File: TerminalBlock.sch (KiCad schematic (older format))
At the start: 2 parts, among them P4 12 Pin Terminal Block, P5 3 Pin TB

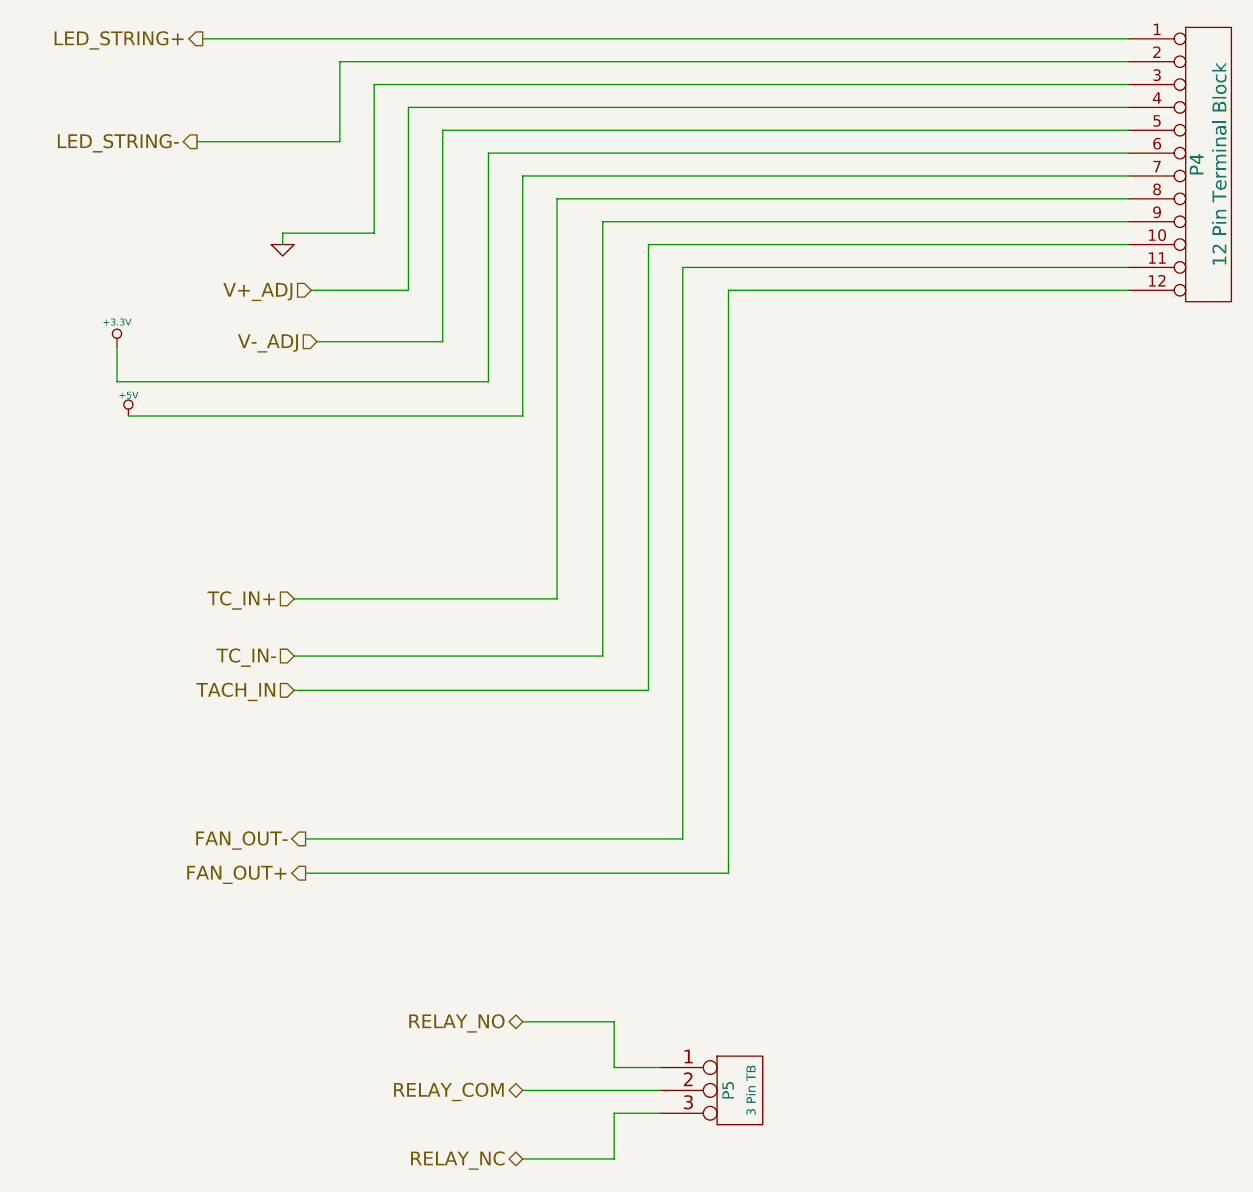
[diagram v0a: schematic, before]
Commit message: Layout Work Session 2
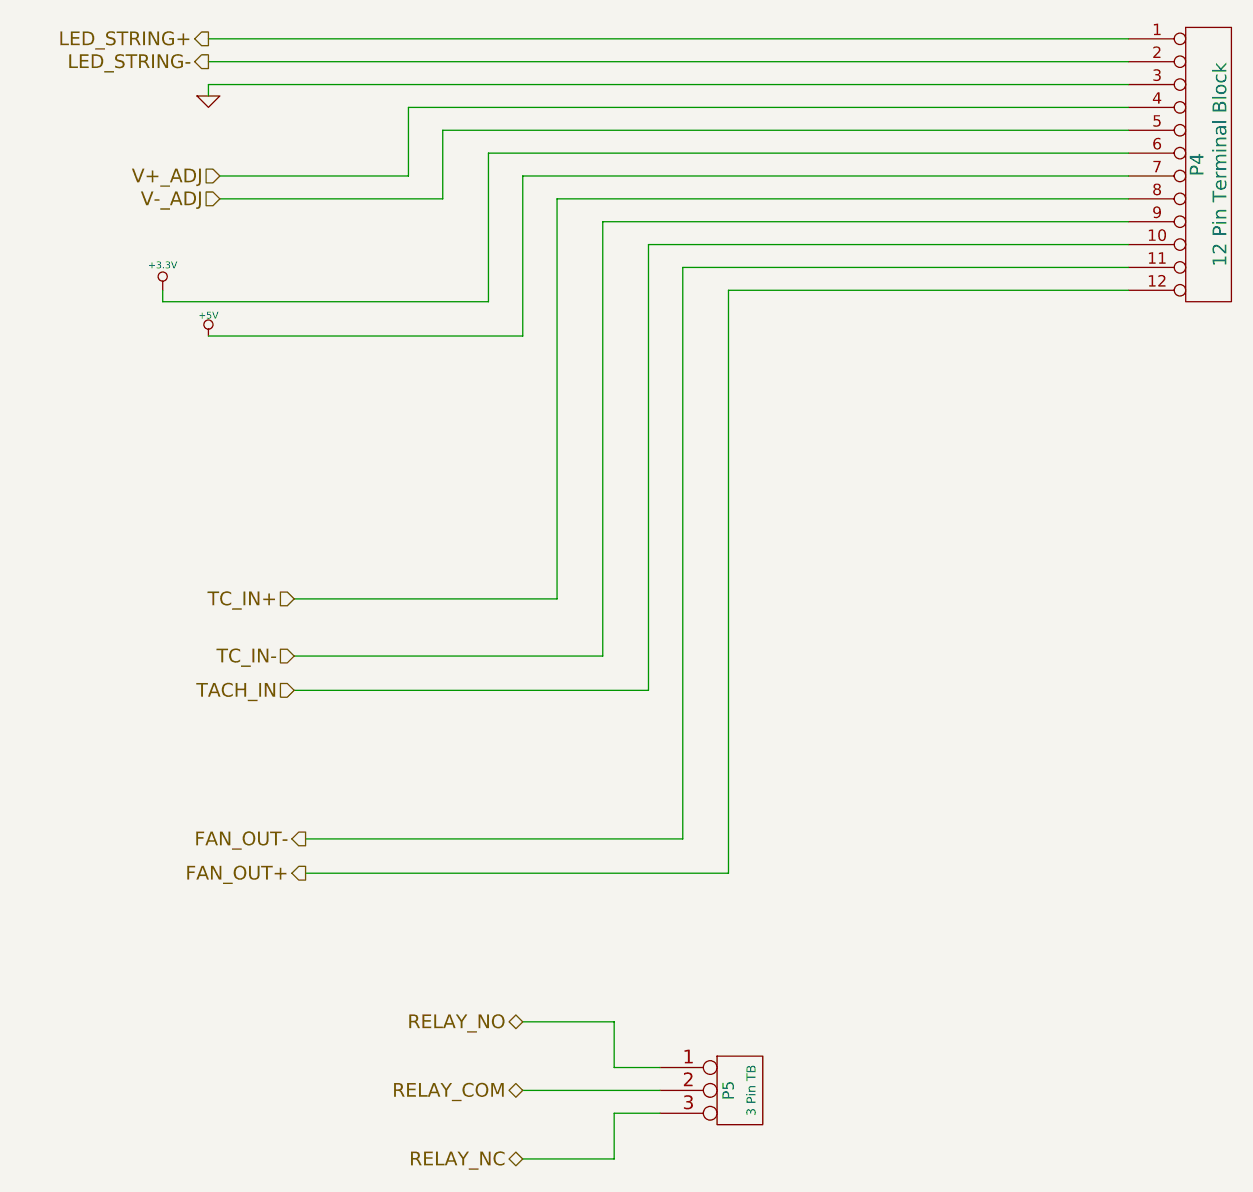
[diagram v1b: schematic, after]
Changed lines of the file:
@@
 LIBS:valves
 LIBS:BenchBuddy
+LIBS:arduino_shieldsNCL
 LIBS:BenchBuddy-cache
 EELAYER 24 0
@@
 Comment4 ""
 $EndDescr
-Text HLabel 1925 2000 0    60   Input ~ 0
+Text HLabel 1525 1500 0    60   Input ~ 0
 V+_ADJ
-Text HLabel 1950 2225 0    60   Input ~ 0
+Text HLabel 1525 1600 0    60   Input ~ 0
 V-_ADJ
 Text HLabel 1900 4550 0    60   Output ~ 0
@@
 Text HLabel 1850 3750 0    60   Input ~ 0
 TACH_IN
-Text HLabel 1450 900  0    60   Output ~ 0
+Text HLabel 1475 900  0    60   Output ~ 0
 LED_STRING+
-Text HLabel 1425 1350 0    60   Output ~ 0
+Text HLabel 1475 1000 0    60   Output ~ 0
 LED_STRING-
 Text HLabel 1850 3350 0    60   Input ~ 0
@@
 RELAY_NC
 $Comp
-L +3.3V #PWR47
+L +3.3V #PWR041
 U 1 1 523FFDA7
-P 1075 2250
-F 0 "#PWR47" H 1075 2210 30  0001 C CNN
-F 1 "+3.3V" H 1075 2360 30  0000 C CNN
-F 2 "~" H 1075 2250 60  0000 C CNN
-F 3 "~" H 1075 2250 60  0000 C CNN
-	1    1075 2250
+P 1275 2000
+F 0 "#PWR041" H 1275 1960 30  0001 C CNN
+F 1 "+3.3V" H 1275 2110 30  0000 C CNN
+F 2 "~" H 1275 2000 60  0000 C CNN
+F 3 "~" H 1275 2000 60  0000 C CNN
+	1    1275 2000
 	1    0    0    -1
 $EndComp
 $Comp
-L +5V #PWR48
+L +5V #PWR042
 U 1 1 523FFDB6
-P 1125 2550
-F 0 "#PWR48" H 1125 2640 20  0001 C CNN
-F 1 "+5V" H 1125 2640 30  0000 C CNN
-F 2 "~" H 1125 2550 60  0000 C CNN
-F 3 "~" H 1125 2550 60  0000 C CNN
-	1    1125 2550
+P 1475 2200
+F 0 "#PWR042" H 1475 2290 20  0001 C CNN
+F 1 "+5V" H 1475 2290 30  0000 C CNN
+F 2 "~" H 1475 2200 60  0000 C CNN
+F 3 "~" H 1475 2200 60  0000 C CNN
+	1    1475 2200
 	1    0    0    -1
 $EndComp
@@
 $EndComp
 Wire Wire Line
-	1450 900  5500 900
+	1475 1000 5500 1000
 Wire Wire Line
-	1425 1350 2050 1350
+	1475 1100 5500 1100
 Wire Wire Line
-	2050 1350 2050 1000
+	1475 1100 1475 1150
 Wire Wire Line
-	2050 1000 5500 1000
-Wire Wire Line
-	2200 1100 5500 1100
-Wire Wire Line
-	2200 1100 2200 1750
-Wire Wire Line
-	1800 1750 1800 1800
-Wire Wire Line
-	2350 2000 2350 1200
+	2350 1500 2350 1200
 Wire Wire Line
 	2350 1200 5500 1200
@@
 	5500 1300 2500 1300
 Wire Wire Line
-	2500 1300 2500 2225
+	2500 1300 2500 1600
 Wire Wire Line
-	2700 2400 2700 1400
+	2700 2050 2700 1400
 Wire Wire Line
 	2700 1400 5500 1400
@@
 	1850 3750 3400 3750
 Wire Wire Line
-	2850 2550 2850 1500
+	2850 2200 2850 1500
 Wire Wire Line
 	2850 1500 5500 1500
@@
 	3250 5800 2850 5800
 Wire Wire Line
-	1125 2550 2850 2550
+	1475 2200 2850 2200
 Wire Wire Line
-	2700 2400 1075 2400
+	2700 2050 1275 2050
 Wire Wire Line
-	1075 2400 1075 2250
+	1275 2050 1275 2000
 Wire Wire Line
-	2500 2225 1950 2225
+	2500 1600 1525 1600
 Wire Wire Line
-	1925 2000 2350 2000
+	1525 1500 2350 1500
 $Comp
-L GND #PWR49
+L GND #PWR043
 U 1 1 523FFDC5
-P 1800 1800
-F 0 "#PWR49" H 1800 1800 30  0001 C CNN
-F 1 "GND" H 1800 1730 30  0001 C CNN
-F 2 "~" H 1800 1800 60  0000 C CNN
-F 3 "~" H 1800 1800 60  0000 C CNN
-	1    1800 1800
+P 1475 1150
+F 0 "#PWR043" H 1475 1150 30  0001 C CNN
+F 1 "GND" H 1475 1080 30  0001 C CNN
+F 2 "~" H 1475 1150 60  0000 C CNN
+F 3 "~" H 1475 1150 60  0000 C CNN
+	1    1475 1150
 	1    0    0    -1
 $EndComp
 Wire Wire Line
-	2200 1750 1800 1750
-Wire Wire Line
-	1750 900  1750 900
+	1475 900  5500 900
 $EndSCHEMATC

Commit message: Layout Work Session 4
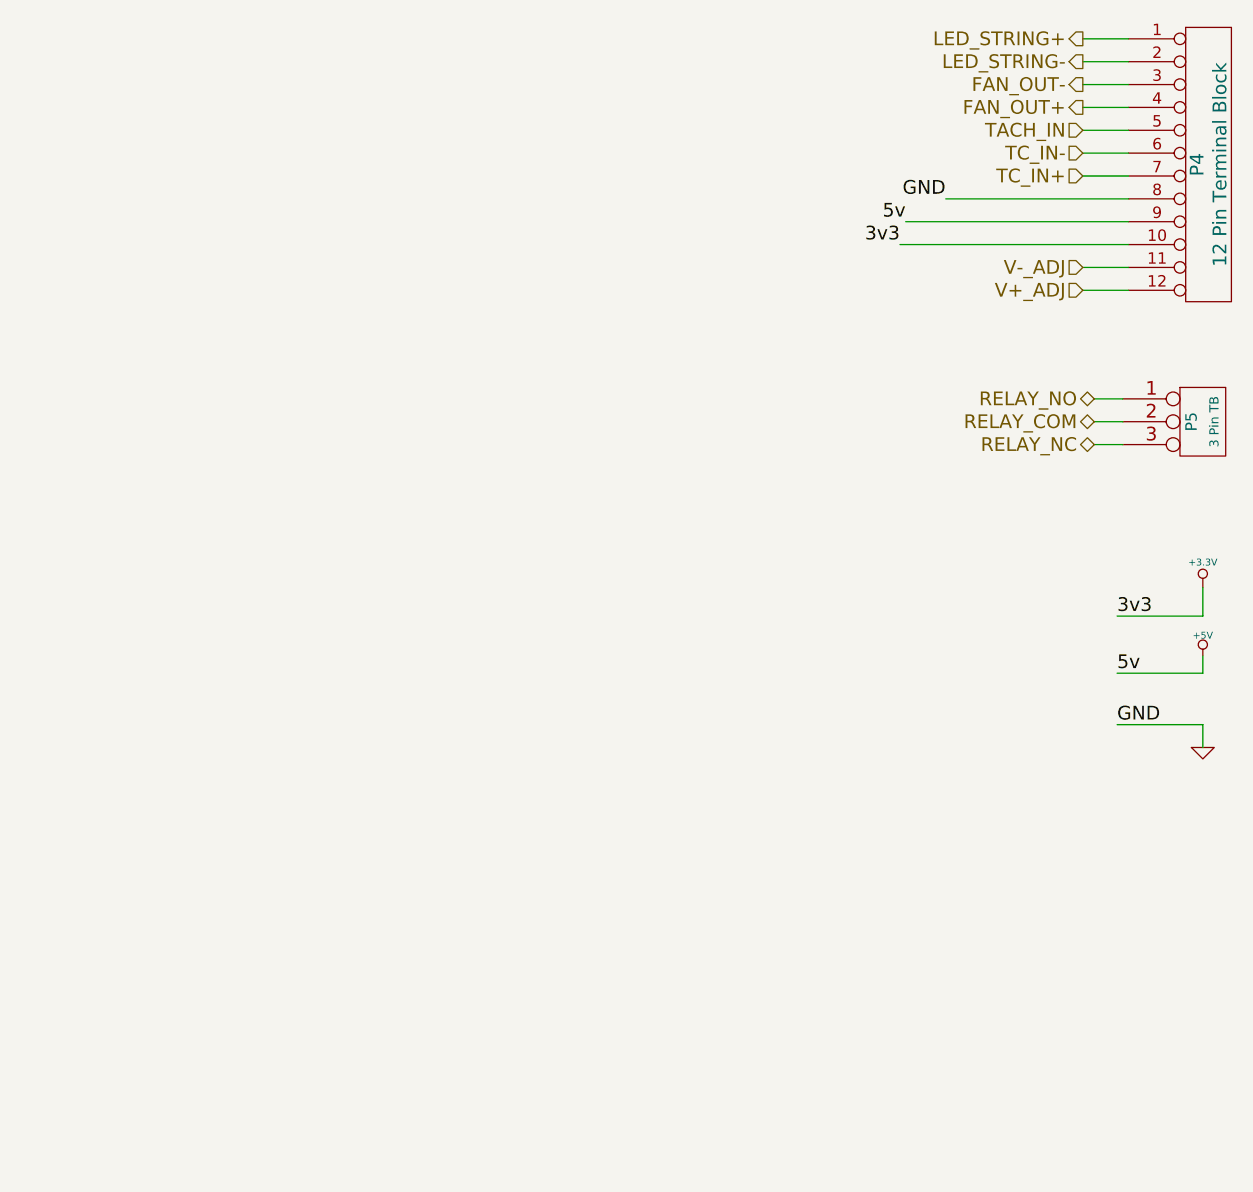
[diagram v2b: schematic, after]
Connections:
- net +3.3V: now also P4.10 (P10); no longer P4.6 (P6)
- net +5V: now also P4.9 (P9); no longer P4.7 (P7)
- net FAN_OUT+: now also P4.4 (P4); no longer P4.12 (P12)
- net FAN_OUT-: now also P4.3 (P3); no longer P4.11 (P11)
- net GND: now also P4.8 (P8); no longer P4.3 (P3)
- net TACH_IN: now also P4.5 (P5); no longer P4.10 (P10)
- net TC_IN+: now also P4.7 (P7); no longer P4.8 (P8)
- net TC_IN-: now also P4.6 (P6); no longer P4.9 (P9)
- net V+_ADJ: now also P4.12 (P12); no longer P4.4 (P4)
- net V-_ADJ: now also P4.11 (P11); no longer P4.5 (P5)
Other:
- moved on the sheet: P5
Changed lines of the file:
@@
 Comment4 ""
 $EndDescr
-Text HLabel 1525 1500 0    60   Input ~ 0
+Text HLabel 5300 2000 0    60   Input ~ 0
 V+_ADJ
-Text HLabel 1525 1600 0    60   Input ~ 0
+Text HLabel 5300 1900 0    60   Input ~ 0
 V-_ADJ
-Text HLabel 1900 4550 0    60   Output ~ 0
+Text HLabel 5300 1200 0    60   Output ~ 0
 FAN_OUT+
-Text HLabel 1900 4400 0    60   Output ~ 0
+Text HLabel 5300 1100 0    60   Output ~ 0
 FAN_OUT-
-Text HLabel 1850 3750 0    60   Input ~ 0
+Text HLabel 5300 1300 0    60   Input ~ 0
 TACH_IN
-Text HLabel 1475 900  0    60   Output ~ 0
+Text HLabel 5300 900  0    60   Output ~ 0
 LED_STRING+
-Text HLabel 1475 1000 0    60   Output ~ 0
+Text HLabel 5300 1000 0    60   Output ~ 0
 LED_STRING-
-Text HLabel 1850 3350 0    60   Input ~ 0
+Text HLabel 5300 1500 0    60   Input ~ 0
 TC_IN+
-Text HLabel 1850 3600 0    60   Input ~ 0
+Text HLabel 5300 1400 0    60   Input ~ 0
 TC_IN-
-Text HLabel 2850 5500 0    60   BiDi ~ 0
+Text HLabel 5350 2575 0    60   BiDi ~ 0
 RELAY_COM
-Text HLabel 2850 5200 0    60   BiDi ~ 0
+Text HLabel 5350 2475 0    60   BiDi ~ 0
 RELAY_NO
-Text HLabel 2850 5800 0    60   BiDi ~ 0
+Text HLabel 5350 2675 0    60   BiDi ~ 0
 RELAY_NC
 $Comp
-L +3.3V #PWR041
+L +3.3V #PWR038
 U 1 1 523FFDA7
-P 1275 2000
-F 0 "#PWR041" H 1275 1960 30  0001 C CNN
-F 1 "+3.3V" H 1275 2110 30  0000 C CNN
-F 2 "~" H 1275 2000 60  0000 C CNN
-F 3 "~" H 1275 2000 60  0000 C CNN
-	1    1275 2000
+P 5825 3300
+F 0 "#PWR038" H 5825 3260 30  0001 C CNN
+F 1 "+3.3V" H 5825 3410 30  0000 C CNN
+F 2 "~" H 5825 3300 60  0000 C CNN
+F 3 "~" H 5825 3300 60  0000 C CNN
+	1    5825 3300
 	1    0    0    -1
 $EndComp
 $Comp
-L +5V #PWR042
+L +5V #PWR039
 U 1 1 523FFDB6
-P 1475 2200
-F 0 "#PWR042" H 1475 2290 20  0001 C CNN
-F 1 "+5V" H 1475 2290 30  0000 C CNN
-F 2 "~" H 1475 2200 60  0000 C CNN
-F 3 "~" H 1475 2200 60  0000 C CNN
-	1    1475 2200
+P 5825 3600
+F 0 "#PWR039" H 5825 3690 20  0001 C CNN
+F 1 "+5V" H 5825 3690 30  0000 C CNN
+F 2 "~" H 5825 3600 60  0000 C CNN
+F 3 "~" H 5825 3600 60  0000 C CNN
+	1    5825 3600
 	1    0    0    -1
 $EndComp
@@
 	1    0    0    -1
 $EndComp
-Wire Wire Line
-	1475 1000 5500 1000
-Wire Wire Line
-	1475 1100 5500 1100
-Wire Wire Line
-	1475 1100 1475 1150
-Wire Wire Line
-	2350 1500 2350 1200
-Wire Wire Line
-	2350 1200 5500 1200
-Wire Wire Line
-	5500 1300 2500 1300
-Wire Wire Line
-	2500 1300 2500 1600
-Wire Wire Line
-	2700 2050 2700 1400
-Wire Wire Line
-	2700 1400 5500 1400
-Wire Wire Line
-	1850 3350 3000 3350
-Wire Wire Line
-	1850 3600 3200 3600
-Wire Wire Line
-	1850 3750 3400 3750
-Wire Wire Line
-	2850 2200 2850 1500
-Wire Wire Line
-	2850 1500 5500 1500
-Wire Wire Line
-	5500 1600 3000 1600
-Wire Wire Line
-	3000 1600 3000 3350
-Wire Wire Line
-	3200 3600 3200 1700
-Wire Wire Line
-	3200 1700 5500 1700
-Wire Wire Line
-	5500 1800 3400 1800
-Wire Wire Line
-	3400 1800 3400 3750
-Wire Wire Line
-	1900 4400 3550 4400
-Wire Wire Line
-	3550 4400 3550 1900
-Wire Wire Line
-	3550 1900 5500 1900
-Wire Wire Line
-	5500 2000 3750 2000
-Wire Wire Line
-	3750 2000 3750 4550
-Wire Wire Line
-	3750 4550 1900 4550
 $Comp
 L CONN_3 P5
 U 1 1 5258AA07
-P 3800 5500
-F 0 "P5" V 3750 5500 50  0000 C CNN
-F 1 "3 Pin TB" V 3850 5500 40  0000 C CNN
-F 2 "" H 3800 5500 60  0000 C CNN
-F 3 "" H 3800 5500 60  0000 C CNN
-F 4 "Phoenix" H 3800 5500 60  0001 C CNN "MFG Name"
-F 5 "1935174" H 3800 5500 60  0001 C CNN "MFG Part Number"
-	1    3800 5500
+P 5825 2575
+F 0 "P5" V 5775 2575 50  0000 C CNN
+F 1 "3 Pin TB" V 5875 2575 40  0000 C CNN
+F 2 "" H 5825 2575 60  0000 C CNN
+F 3 "" H 5825 2575 60  0000 C CNN
+F 4 "Phoenix" H 5825 2575 60  0001 C CNN "MFG Name"
+F 5 "1935174" H 5825 2575 60  0001 C CNN "MFG Part Number"
+	1    5825 2575
 	1    0    0    -1
 $EndComp
 Wire Wire Line
-	3450 5500 2850 5500
-Wire Wire Line
-	2850 5200 3250 5200
-Wire Wire Line
-	3250 5200 3250 5400
-Wire Wire Line
-	3250 5400 3450 5400
-Wire Wire Line
-	3450 5600 3250 5600
-Wire Wire Line
-	3250 5600 3250 5800
-Wire Wire Line
-	3250 5800 2850 5800
-Wire Wire Line
-	1475 2200 2850 2200
-Wire Wire Line
-	2700 2050 1275 2050
-Wire Wire Line
-	1275 2050 1275 2000
-Wire Wire Line
-	2500 1600 1525 1600
-Wire Wire Line
-	1525 1500 2350 1500
+	5475 2575 5350 2575
 $Comp
-L GND #PWR043
+L GND #PWR040
 U 1 1 523FFDC5
-P 1475 1150
-F 0 "#PWR043" H 1475 1150 30  0001 C CNN
-F 1 "GND" H 1475 1080 30  0001 C CNN
-F 2 "~" H 1475 1150 60  0000 C CNN
-F 3 "~" H 1475 1150 60  0000 C CNN
-	1    1475 1150
+P 5825 4000
+F 0 "#PWR040" H 5825 4000 30  0001 C CNN
+F 1 "GND" H 5825 3930 30  0001 C CNN
+F 2 "~" H 5825 4000 60  0000 C CNN
+F 3 "~" H 5825 4000 60  0000 C CNN
+	1    5825 4000
 	1    0    0    -1
 $EndComp
 Wire Wire Line
-	1475 900  5500 900
+	5350 2475 5475 2475
+Wire Wire Line
+	5350 2675 5475 2675
+Wire Wire Line
+	5825 3300 5825 3425
+Wire Wire Line
+	5825 3425 5450 3425
+Text Label 5450 3425 0    60   ~ 0
+3v3
+Wire Wire Line
+	5825 3600 5825 3675
+Wire Wire Line
+	5825 3675 5450 3675
+Wire Wire Line
+	5825 4000 5825 3900
+Wire Wire Line
+	5825 3900 5450 3900
+Text Label 5450 3675 0    60   ~ 0
+5v
+Text Label 5450 3900 0    60   ~ 0
+GND
+Wire Wire Line
+	5300 2000 5500 2000
+Wire Wire Line
+	5500 1900 5300 1900
+Wire Wire Line
+	4500 1800 5500 1800
+Wire Wire Line
+	4525 1700 5500 1700
+Wire Wire Line
+	4700 1600 5500 1600
+Wire Wire Line
+	5500 1300 5300 1300
+Wire Wire Line
+	5500 900  5300 900
+Wire Wire Line
+	5300 1000 5500 1000
+Wire Wire Line
+	5500 1200 5300 1200
+Wire Wire Line
+	5500 1100 5300 1100
+Wire Wire Line
+	5500 1400 5300 1400
+Wire Wire Line
+	5500 1500 5300 1500
+Text Label 4500 1800 2    60   ~ 0
+3v3
+Text Label 4525 1700 2    60   ~ 0
+5v
+Text Label 4700 1600 2    60   ~ 0
+GND
 $EndSCHEMATC
